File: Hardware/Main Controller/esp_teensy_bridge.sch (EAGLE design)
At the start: 64 parts, among them IC1 BQ79600PWRQ1, Q5 VISHAY_SIS862DN-T1-GE3VISHAY_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, Q6 VISHAY_SIS862DN-T1-GE3VISHAY_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, Q7 VISHAY_SIS862DN-T1-GE3VISHAY_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, Q8 VISHAY_SIS862DN-T1-GE3VISHAY_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, X1 5566-12

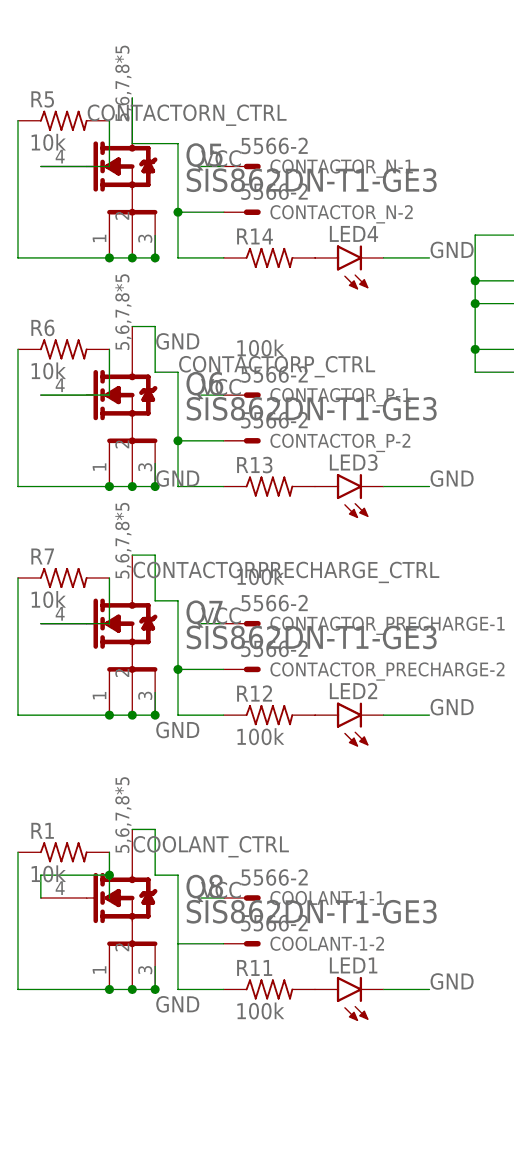
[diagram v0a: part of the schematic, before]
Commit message: Fixed LED issue
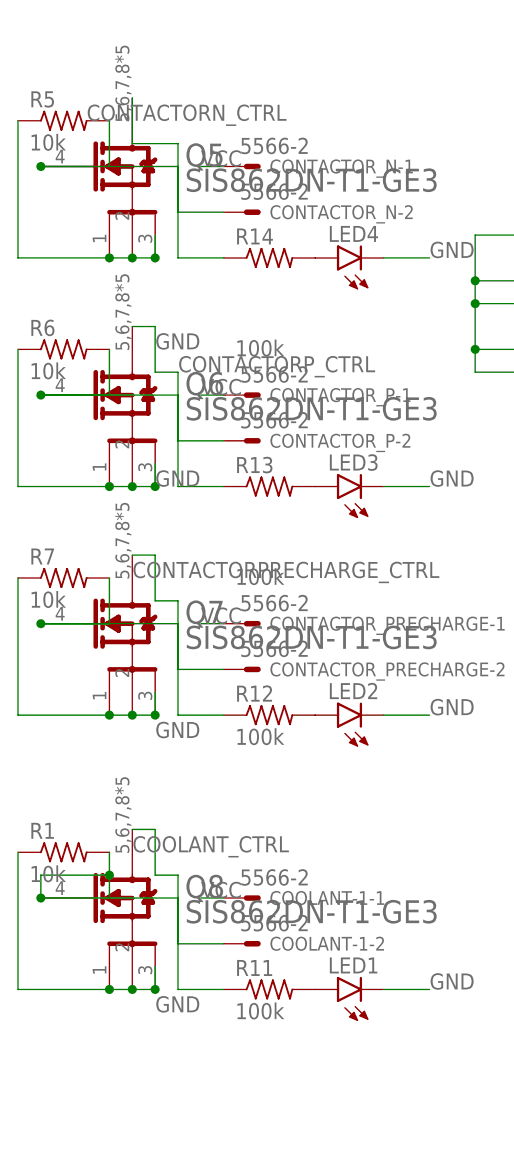
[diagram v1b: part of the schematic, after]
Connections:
- net CONTACTORN_CTRL: now also R14.1
- net CONTACTORPRECHARGE_CTRL: now also R12.1
- net CONTACTORP_CTRL: now also R13.1
- net COOLANT_CTRL: now also R11.1
- net N$12: no longer R12.1
- net N$2: no longer R13.1
- net N$5: no longer R14.1
- net N$6: no longer R11.1
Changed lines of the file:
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@@
 <pinref part="Q5" gate="G$0" pin="G"/>
 <wire x1="-134.62" y1="71.12" x2="-142.24" y2="71.12" width="0.1524" layer="91"/>
+<pinref part="R14" gate="G$1" pin="1"/>
+<wire x1="-127" y1="60.96" x2="-121.92" y2="60.96" width="0.1524" layer="91"/>
+<wire x1="-127" y1="60.96" x2="-127" y2="71.12" width="0.1524" layer="91"/>
+<wire x1="-127" y1="71.12" x2="-142.24" y2="71.12" width="0.1524" layer="91"/>
+<junction x="-142.24" y="71.12"/>
 </segment>
 <segment>
@@
 <pinref part="CONTACTOR_N" gate="-2" pin="S"/>
 <wire x1="-127" y1="66.04" x2="-121.92" y2="66.04" width="0.1524" layer="91"/>
-<pinref part="R14" gate="G$1" pin="1"/>
-<wire x1="-127" y1="66.04" x2="-127" y2="60.96" width="0.1524" layer="91"/>
-<wire x1="-127" y1="60.96" x2="-121.92" y2="60.96" width="0.1524" layer="91"/>
-<junction x="-127" y="66.04"/>
 <pinref part="Q5" gate="G$0" pin="D"/>
 <wire x1="-132.08" y1="78.74" x2="-132.08" y2="73.66" width="0.1524" layer="91"/>
@@
 <wire x1="-127" y1="48.26" x2="-127" y2="40.64" width="0.1524" layer="91"/>
 <wire x1="-127" y1="40.64" x2="-121.92" y2="40.64" width="0.1524" layer="91"/>
-<pinref part="R13" gate="G$1" pin="1"/>
-<wire x1="-127" y1="40.64" x2="-127" y2="35.56" width="0.1524" layer="91"/>
-<wire x1="-127" y1="35.56" x2="-121.92" y2="35.56" width="0.1524" layer="91"/>
-<junction x="-127" y="40.64"/>
 <pinref part="Q6" gate="G$0" pin="D"/>
 <wire x1="-129.54" y1="48.26" x2="-129.54" y2="53.34" width="0.1524" layer="91"/>
@@
 <pinref part="Q6" gate="G$0" pin="G"/>
 <wire x1="-134.62" y1="45.72" x2="-142.24" y2="45.72" width="0.1524" layer="91"/>
+<pinref part="R13" gate="G$1" pin="1"/>
+<wire x1="-127" y1="35.56" x2="-121.92" y2="35.56" width="0.1524" layer="91"/>
+<wire x1="-127" y1="35.56" x2="-127" y2="45.72" width="0.1524" layer="91"/>
+<wire x1="-127" y1="45.72" x2="-142.24" y2="45.72" width="0.1524" layer="91"/>
+<junction x="-142.24" y="45.72"/>
 </segment>
 <segment>
@@
 <pinref part="Q7" gate="G$0" pin="G"/>
 <wire x1="-134.62" y1="20.32" x2="-142.24" y2="20.32" width="0.1524" layer="91"/>
+<pinref part="R12" gate="G$1" pin="1"/>
+<wire x1="-127" y1="10.16" x2="-121.92" y2="10.16" width="0.1524" layer="91"/>
+<wire x1="-127" y1="10.16" x2="-127" y2="20.32" width="0.1524" layer="91"/>
+<wire x1="-127" y1="20.32" x2="-142.24" y2="20.32" width="0.1524" layer="91"/>
+<junction x="-142.24" y="20.32"/>
 </segment>
 <segment>
@@
 <pinref part="CONTACTOR_PRECHARGE" gate="-2" pin="S"/>
 <wire x1="-127" y1="15.24" x2="-121.92" y2="15.24" width="0.1524" layer="91"/>
-<pinref part="R12" gate="G$1" pin="1"/>
-<wire x1="-127" y1="15.24" x2="-127" y2="10.16" width="0.1524" layer="91"/>
-<wire x1="-127" y1="10.16" x2="-121.92" y2="10.16" width="0.1524" layer="91"/>
-<junction x="-127" y="15.24"/>
 <pinref part="Q7" gate="G$0" pin="D"/>
 <wire x1="-129.54" y1="22.86" x2="-129.54" y2="27.94" width="0.1524" layer="91"/>
@@
 <pinref part="COOLANT-1" gate="-2" pin="S"/>
 <wire x1="-121.92" y1="-15.24" x2="-127" y2="-15.24" width="0.1524" layer="91"/>
-<wire x1="-127" y1="-15.24" x2="-127" y2="-20.32" width="0.1524" layer="91"/>
-<wire x1="-127" y1="-20.32" x2="-121.92" y2="-20.32" width="0.1524" layer="91"/>
-<pinref part="R11" gate="G$1" pin="1"/>
 <pinref part="Q8" gate="G$0" pin="D"/>
 <wire x1="-129.54" y1="-7.62" x2="-129.54" y2="-2.54" width="0.1524" layer="91"/>
@@
 <wire x1="-142.24" y1="-7.62" x2="-142.24" y2="-10.16" width="0.1524" layer="91"/>
 <junction x="-134.62" y="-7.62"/>
+<wire x1="-127" y1="-20.32" x2="-121.92" y2="-20.32" width="0.1524" layer="91"/>
+<pinref part="R11" gate="G$1" pin="1"/>
+<wire x1="-127" y1="-20.32" x2="-127" y2="-10.16" width="0.1524" layer="91"/>
+<wire x1="-127" y1="-10.16" x2="-142.24" y2="-10.16" width="0.1524" layer="91"/>
+<junction x="-142.24" y="-10.16"/>
 </segment>
 <segment>
